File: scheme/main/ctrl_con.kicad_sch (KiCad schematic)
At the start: 0 parts

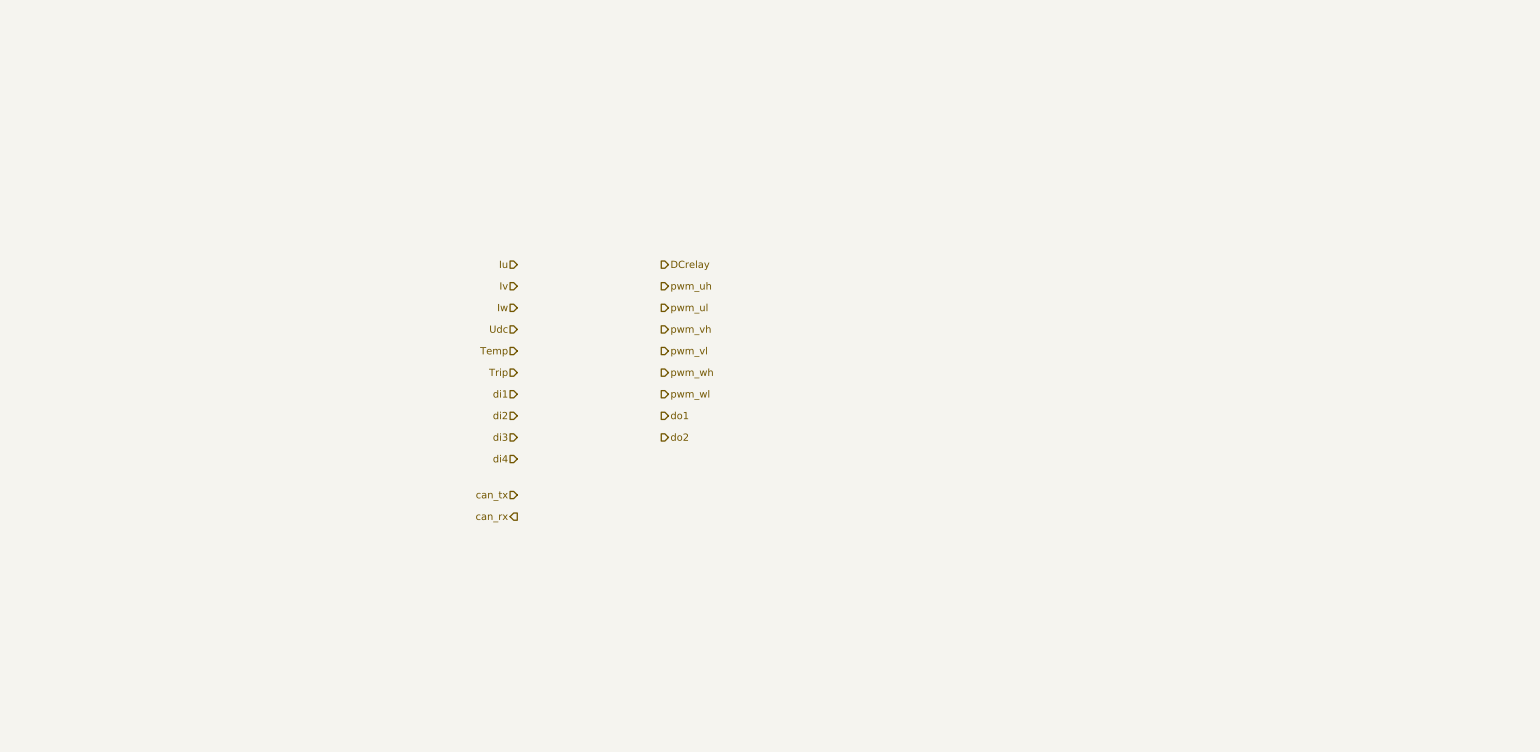
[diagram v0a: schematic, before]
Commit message: boards schematic sheets & more
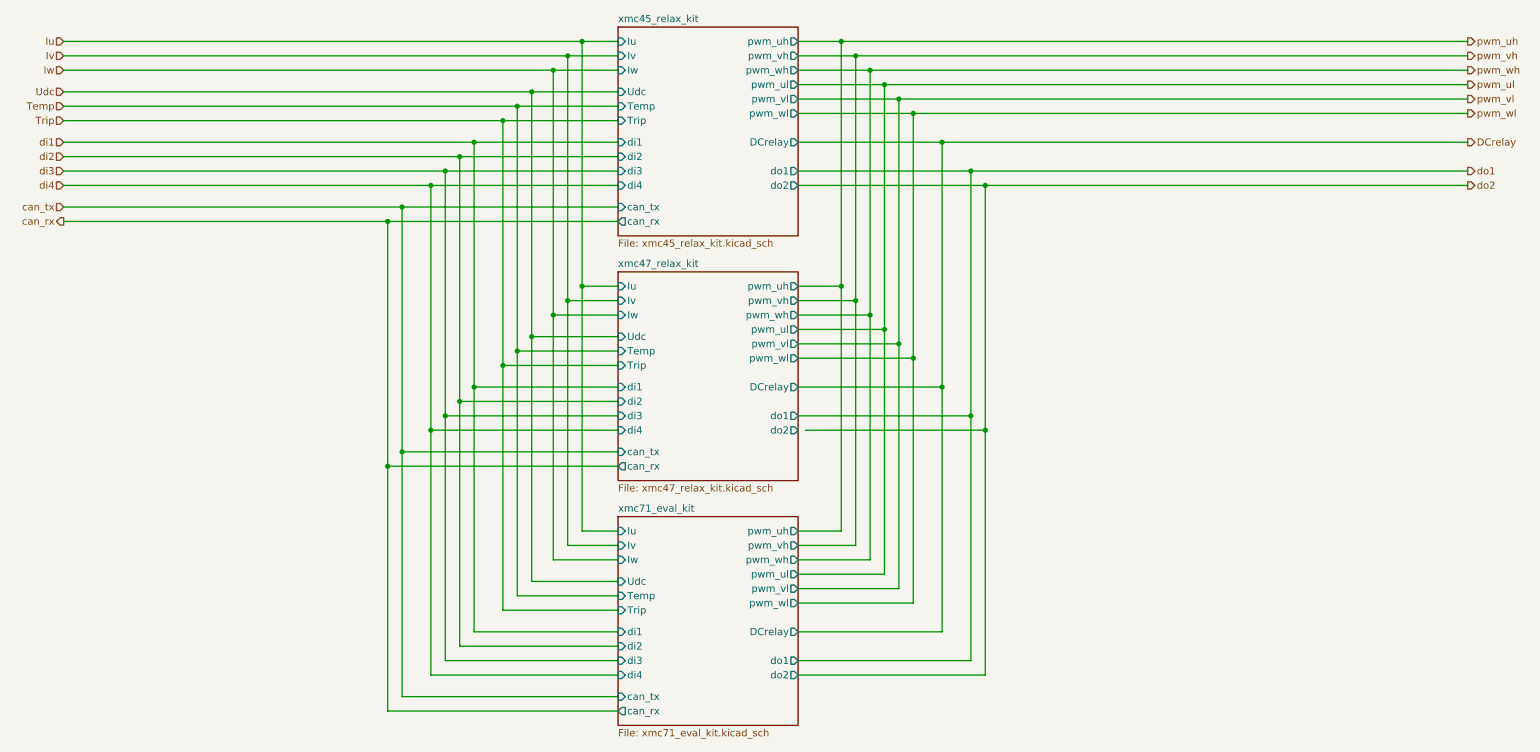
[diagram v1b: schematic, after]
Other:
- added sheet xmc45_relax_kit (xmc45_relax_kit.kicad_sch)
- added sheet xmc47_relax_kit (xmc47_relax_kit.kicad_sch)
- added sheet xmc71_eval_kit (xmc71_eval_kit.kicad_sch)
